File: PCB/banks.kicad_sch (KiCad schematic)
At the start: 8 parts, among them U1 XC7A50T-FGG484, Y3 100MHz

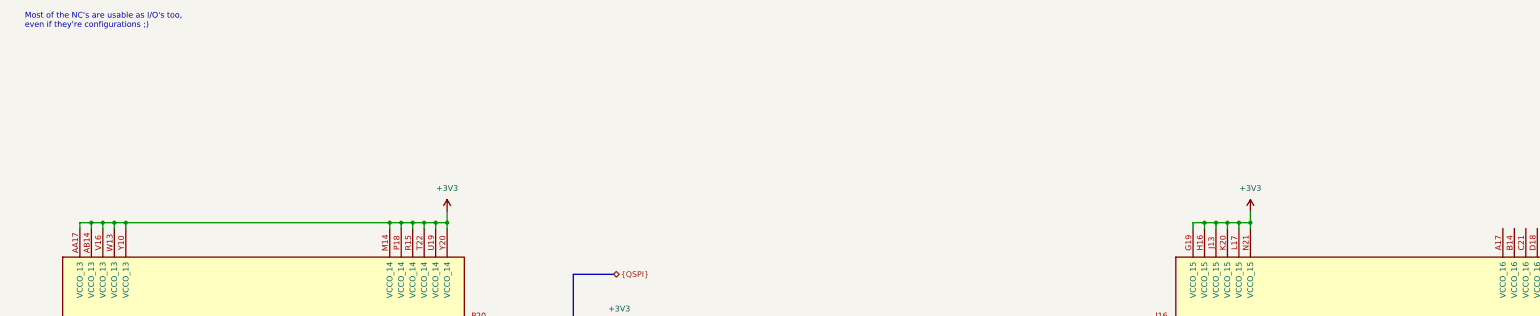
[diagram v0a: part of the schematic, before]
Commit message: forgot to add decouping to my banks
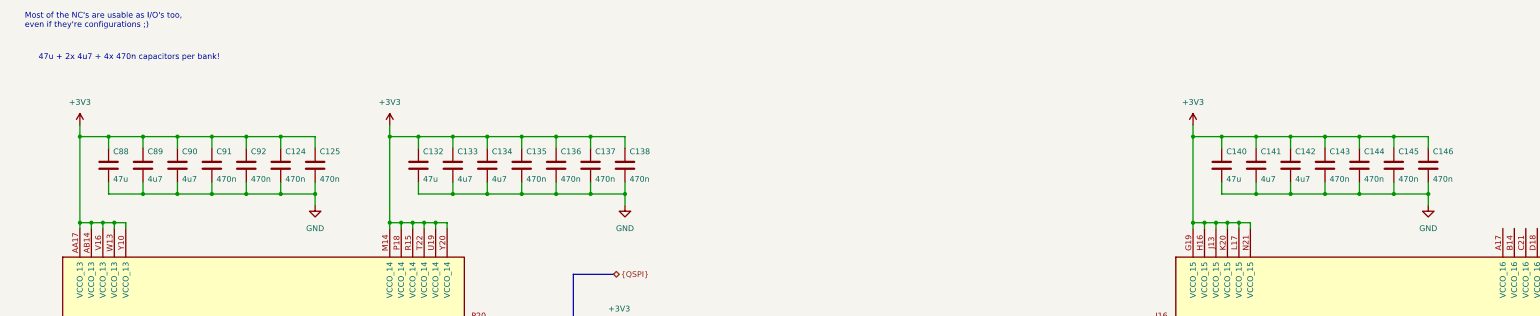
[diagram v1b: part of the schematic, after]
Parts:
- added C124, C125, C135, C136, C137, C138, C143, C144, C145, C146, C91, C92: 470n, Capacitor_SMD:C_0201_0603Metric, symbol Device:C
- added C132, C140, C88: 47u, Capacitor_SMD:C_1206_3216Metric, symbol Device:C
- added C133, C134, C141, C142, C89, C90: 4u7, Capacitor_SMD:C_0603_1608Metric, symbol Device:C
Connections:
- net +3V3: now also C124.1, C125.1, C132.1, C133.1, C134.1, C135.1, C136.1, C137.1, C138.1, C140.1, C141.1, C142.1, C143.1, C144.1, C145.1, C146.1, C88.1, C89.1, C90.1, C91.1, C92.1
- net GND: now also C124.2, C125.2, C132.2, C133.2, C134.2, C135.2, C136.2, C137.2, C138.2, C140.2, C141.2, C142.2, C143.2, C144.2, C145.2, C146.2, C88.2, C89.2, C90.2, C91.2, C92.2
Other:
- note added: "47u + 2x 4u7 + 4x 470n capacitors per bank!"

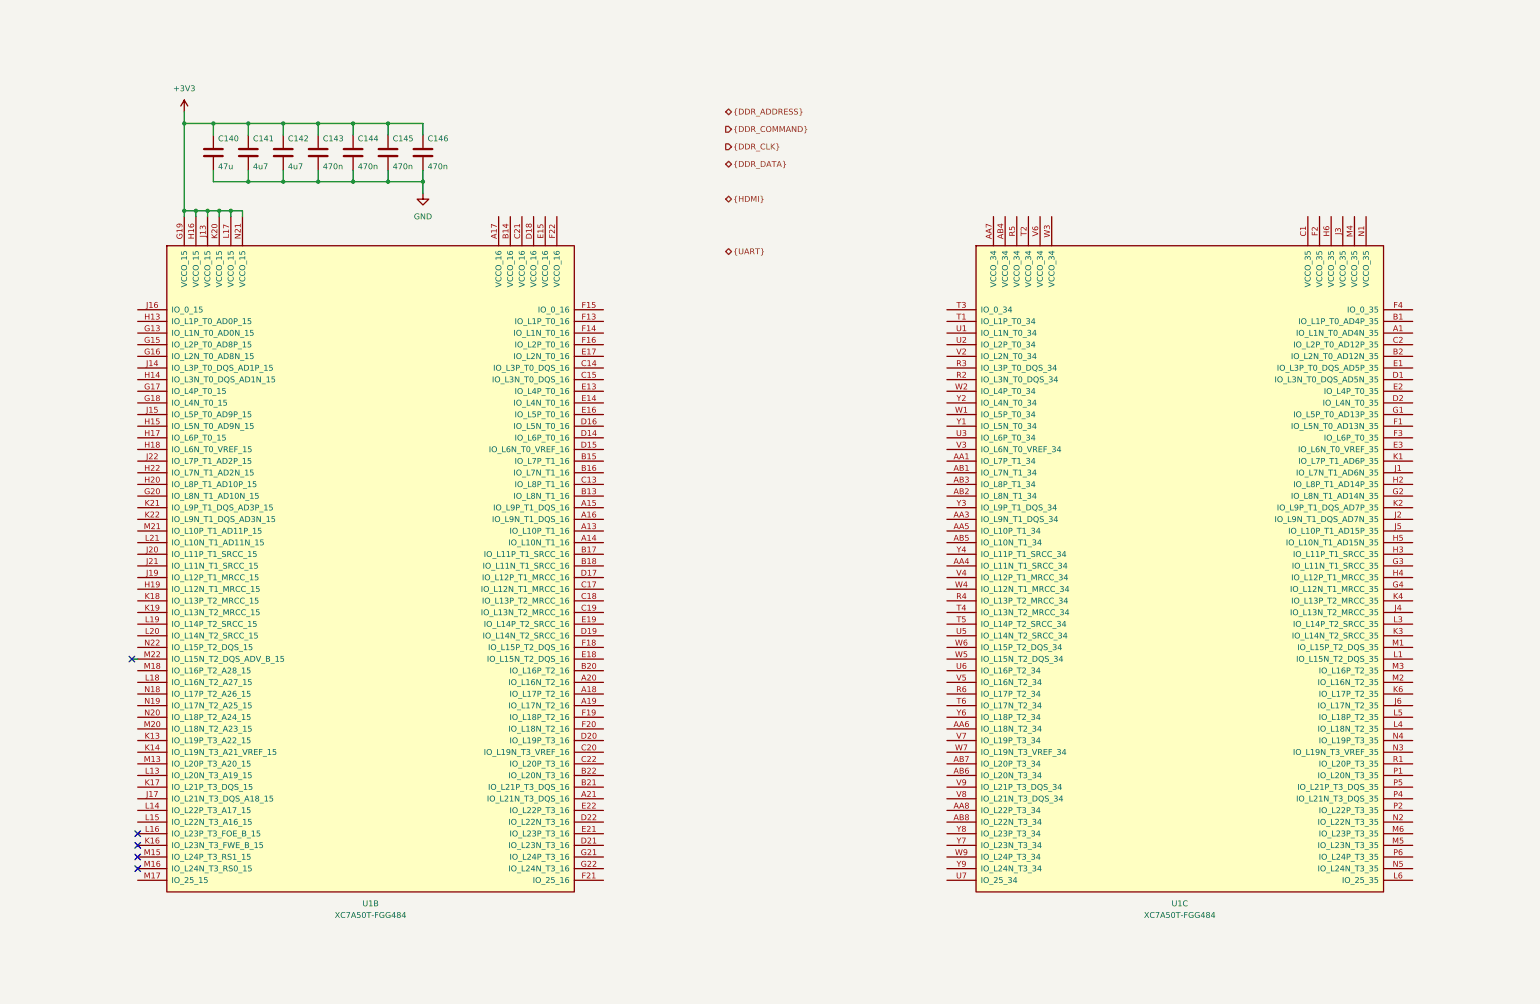
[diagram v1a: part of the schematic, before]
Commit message: wired decoupling to banks 34 and 35
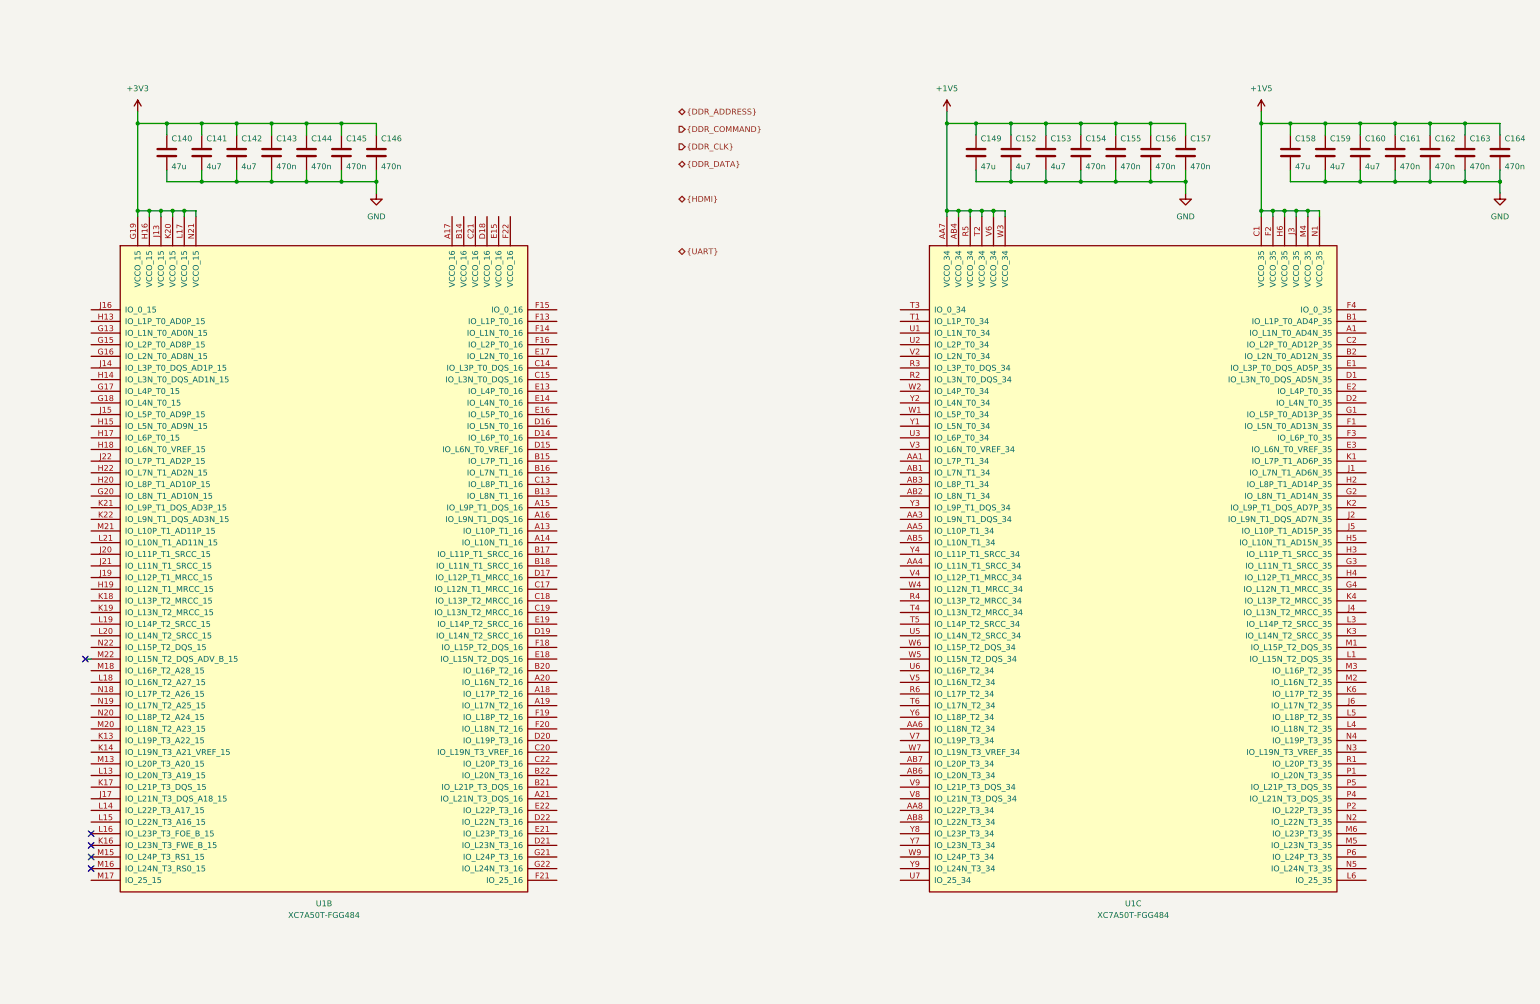
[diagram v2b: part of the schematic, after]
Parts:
- added C149, C158: 47u, Capacitor_SMD:C_1206_3216Metric, symbol Device:C
- added C152, C153, C159, C160: 4u7, Capacitor_SMD:C_0603_1608Metric, symbol Device:C
- added C154, C155, C156, C157, C161, C162, C163, C164: 470n, Capacitor_SMD:C_0201_0603Metric, symbol Device:C
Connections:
- net GND: now also C149.2, C152.2, C153.2, C154.2, C155.2, C156.2, C157.2, C158.2, C159.2, C160.2, C161.2, C162.2, C163.2, C164.2
- net +1V5: now reaches U1.AA7 (VCCO_34)
- net +1V5: now also U1.AB4 (VCCO_34), U1.C1 (VCCO_35), U1.F2 (VCCO_35), U1.H6 (VCCO_35), U1.J3 (VCCO_35), U1.M4 (VCCO_35), U1.N1 (VCCO_35), U1.R5 (VCCO_34), U1.T2 (VCCO_34), U1.V6 (VCCO_34), U1.W3 (VCCO_34), C149.1, C152.1, C153.1, C154.1, C155.1, C156.1, C157.1, C158.1, C159.1, C160.1, C161.1, C162.1, C163.1, C164.1
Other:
- moved on the sheet: C140, C141, C142, C143, C144, C145, C146, U1B, U1C

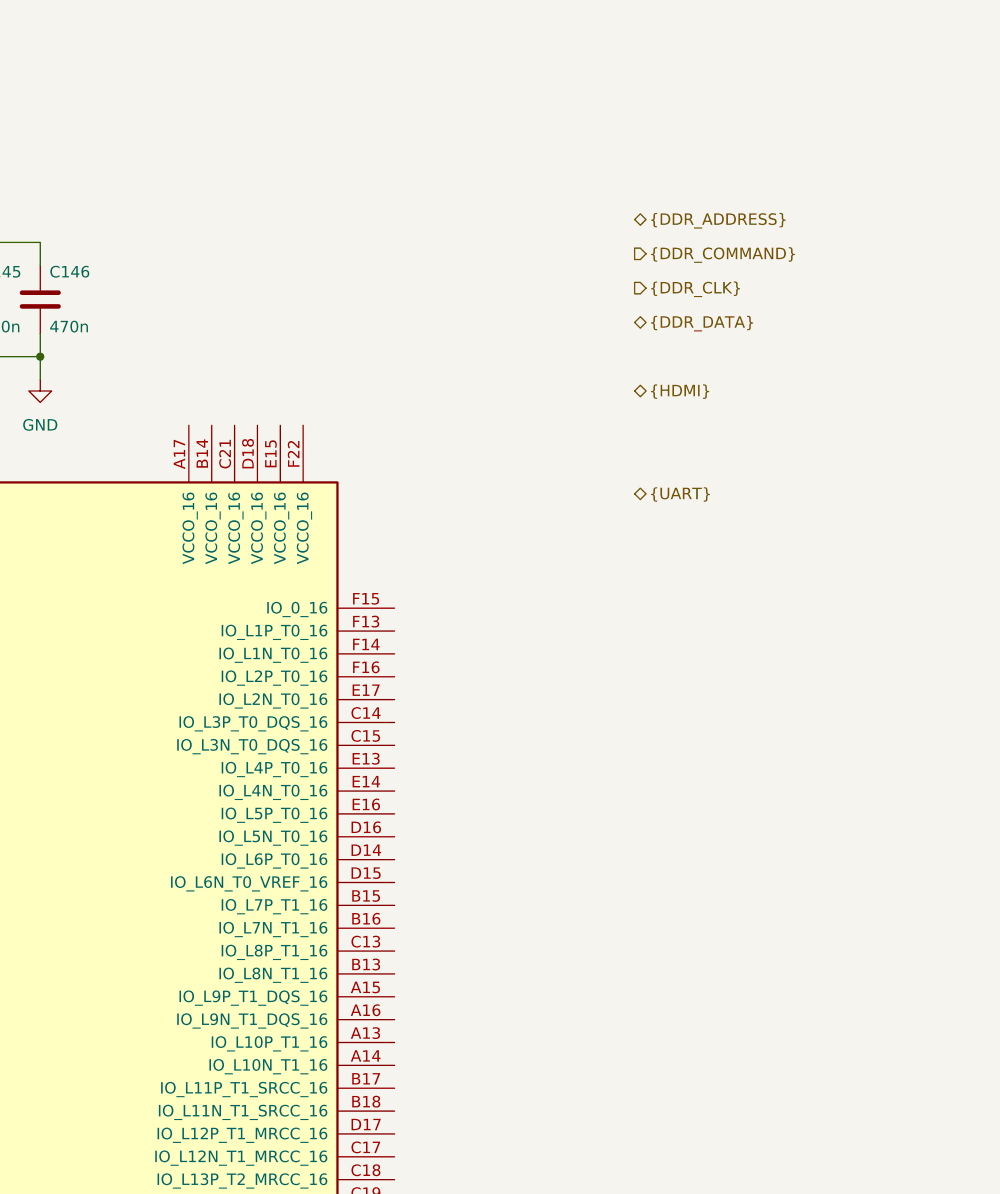
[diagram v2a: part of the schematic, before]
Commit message: wired up bank 16
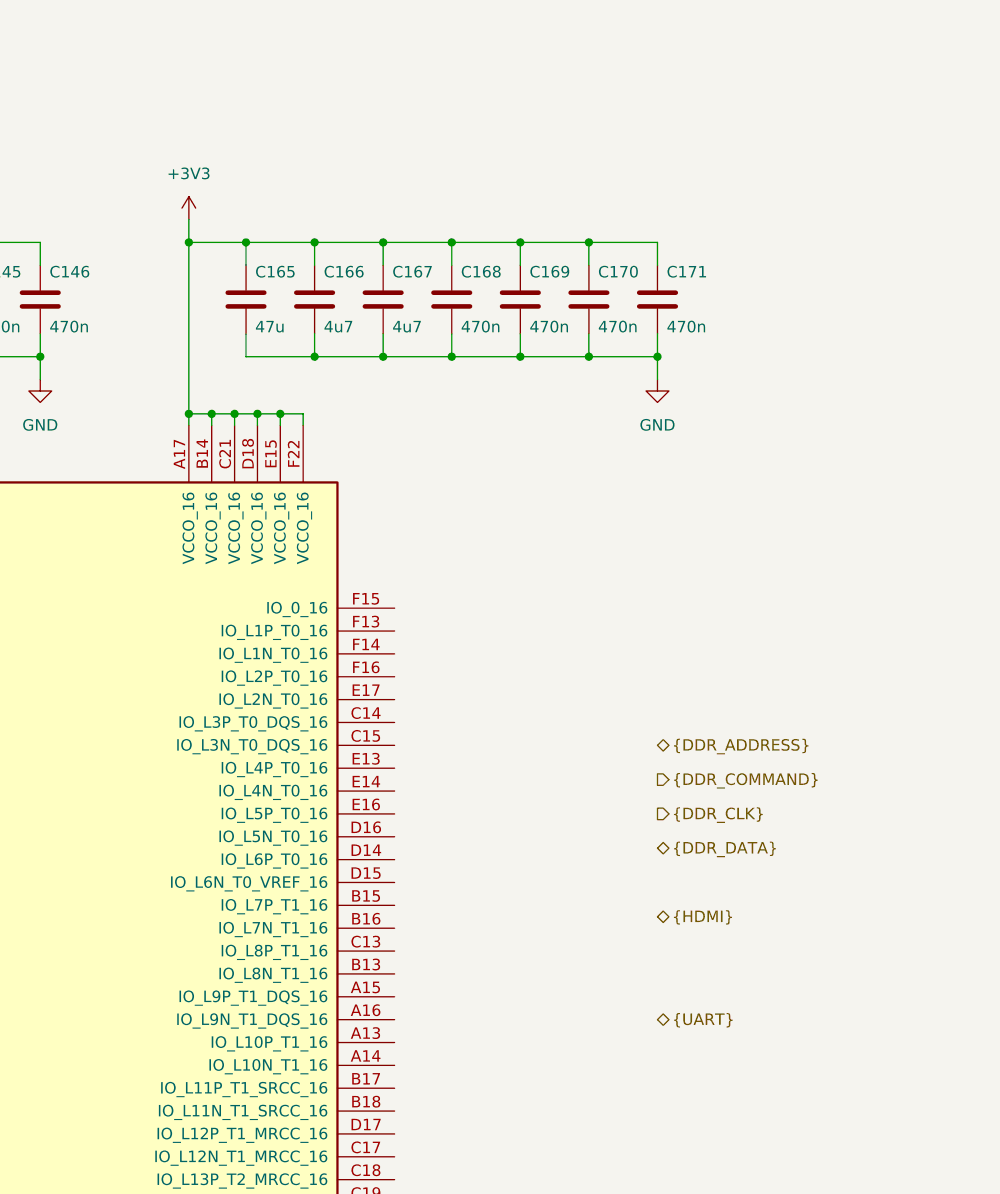
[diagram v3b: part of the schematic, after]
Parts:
- added C165: 47u, Capacitor_SMD:C_1206_3216Metric, symbol Device:C
- added C166, C167: 4u7, Capacitor_SMD:C_0603_1608Metric, symbol Device:C
- added C168, C169, C170, C171: 470n, Capacitor_SMD:C_0201_0603Metric, symbol Device:C
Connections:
- net +3V3: now also U1.A17 (VCCO_16), U1.B14 (VCCO_16), U1.C21 (VCCO_16), U1.D18 (VCCO_16), U1.E15 (VCCO_16), U1.F22 (VCCO_16), C165.1, C166.1, C167.1, C168.1, C169.1, C170.1, C171.1
- net GND: now also C165.2, C166.2, C167.2, C168.2, C169.2, C170.2, C171.2
